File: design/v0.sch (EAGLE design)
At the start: 3 parts

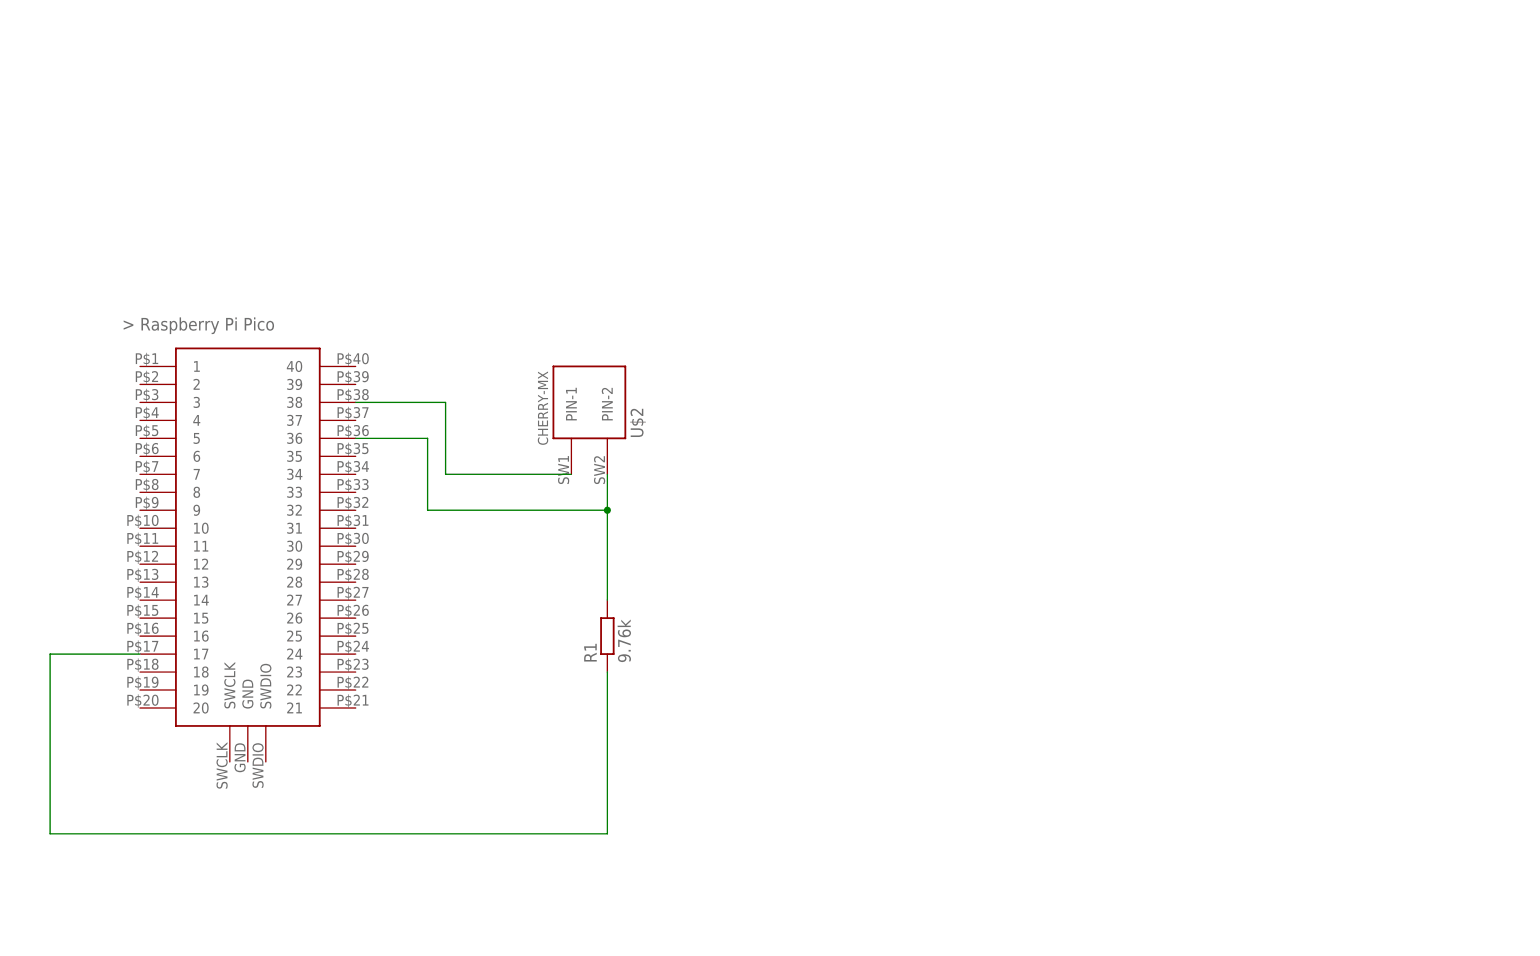
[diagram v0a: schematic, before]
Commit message: Update schematic
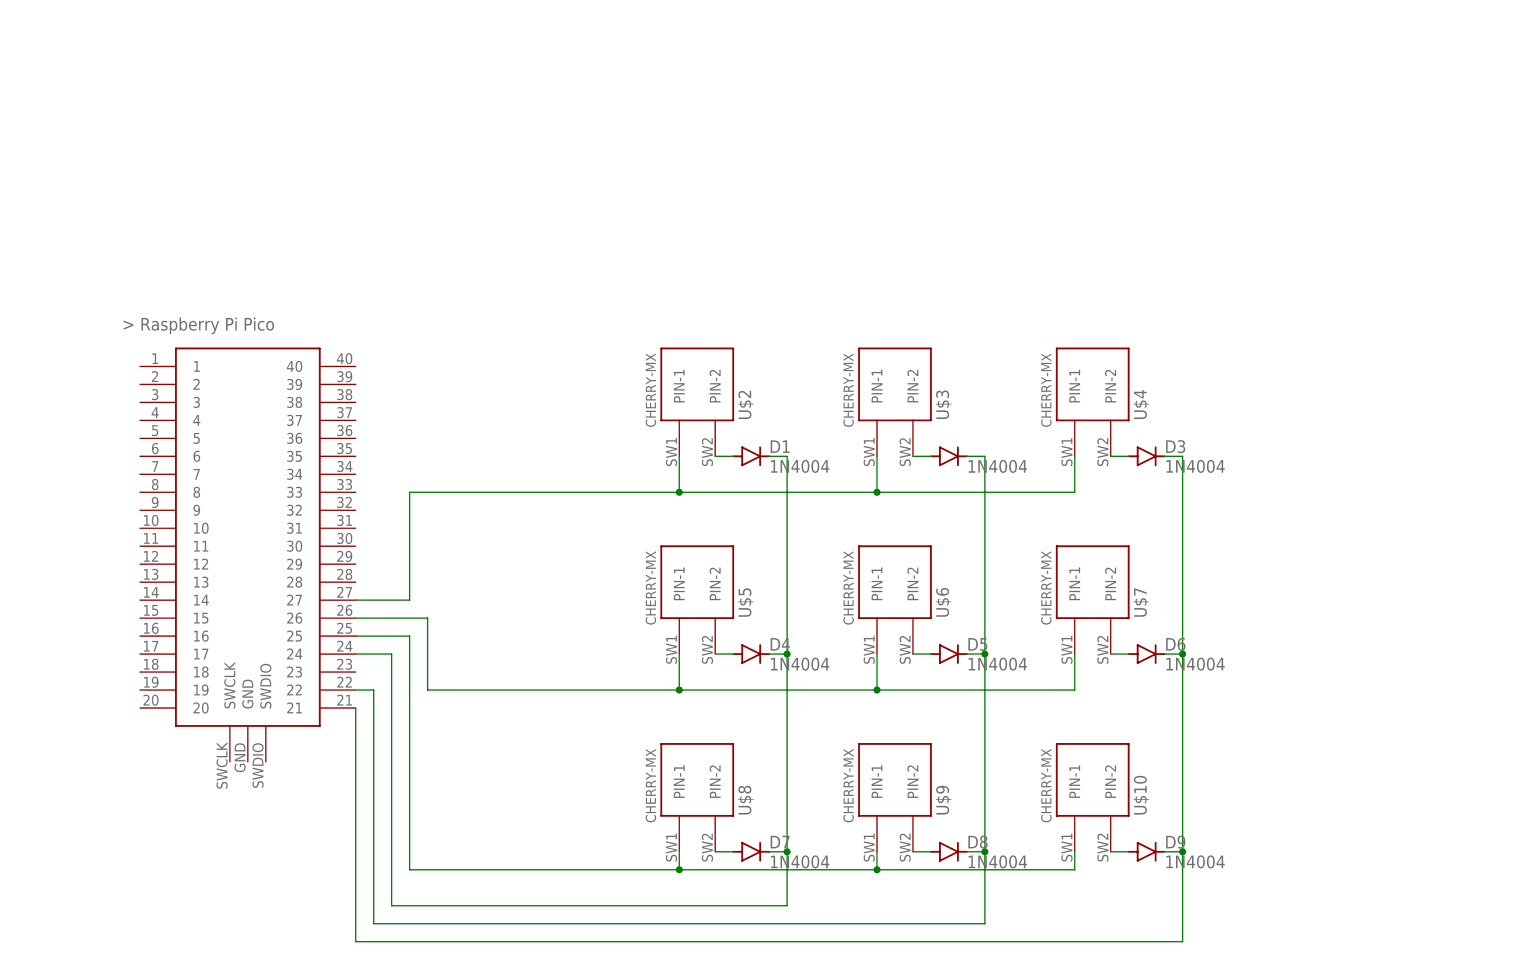
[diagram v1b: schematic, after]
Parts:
- removed R1: 9.76k, rcl:R-EU_0207/10
- added D1, D2, D3, D4, D5, D6, D7, D8, D9: 1N4004, diode:1N4004
- added U$10, U$3, U$4, U$5, U$6, U$7, U$8, U$9: CHERRY-MX, cherrymx:CHERRY-MX
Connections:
- new net N$10: D1.C, D4.C, D7.C, U$1.24
- new net N$11: D2.C, D5.C, D8.C, U$1.22
- new net N$12: D3.C, D6.C, D9.C, U$1.21
- new net N$13: U$1.27, U$2.PIN-1, U$3.PIN-1, U$4.PIN-1
- new net N$14: U$1.26, U$5.PIN-1, U$6.PIN-1, U$7.PIN-1
- new net N$15: U$1.25, U$10.PIN-1, U$8.PIN-1, U$9.PIN-1
- new net N$3: D3.A, U$4.PIN-2
- new net N$5: D5.A, U$6.PIN-2
- new net N$6: D6.A, U$7.PIN-2
- new net N$7: D9.A, U$10.PIN-2
- new net N$8: D8.A, U$9.PIN-2
- new net N$9: D7.A, U$8.PIN-2
- net N$1: now also D1.A, U$2.PIN-2; no longer U$1.38, U$2.PIN-1
- net N$2: now also D2.A, U$3.PIN-2; no longer R1.2, U$1.36, U$2.PIN-2
- net N$4: now also D4.A, U$5.PIN-2; no longer R1.1, U$1.17
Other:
- moved on the sheet: U$2

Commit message: Update schematic
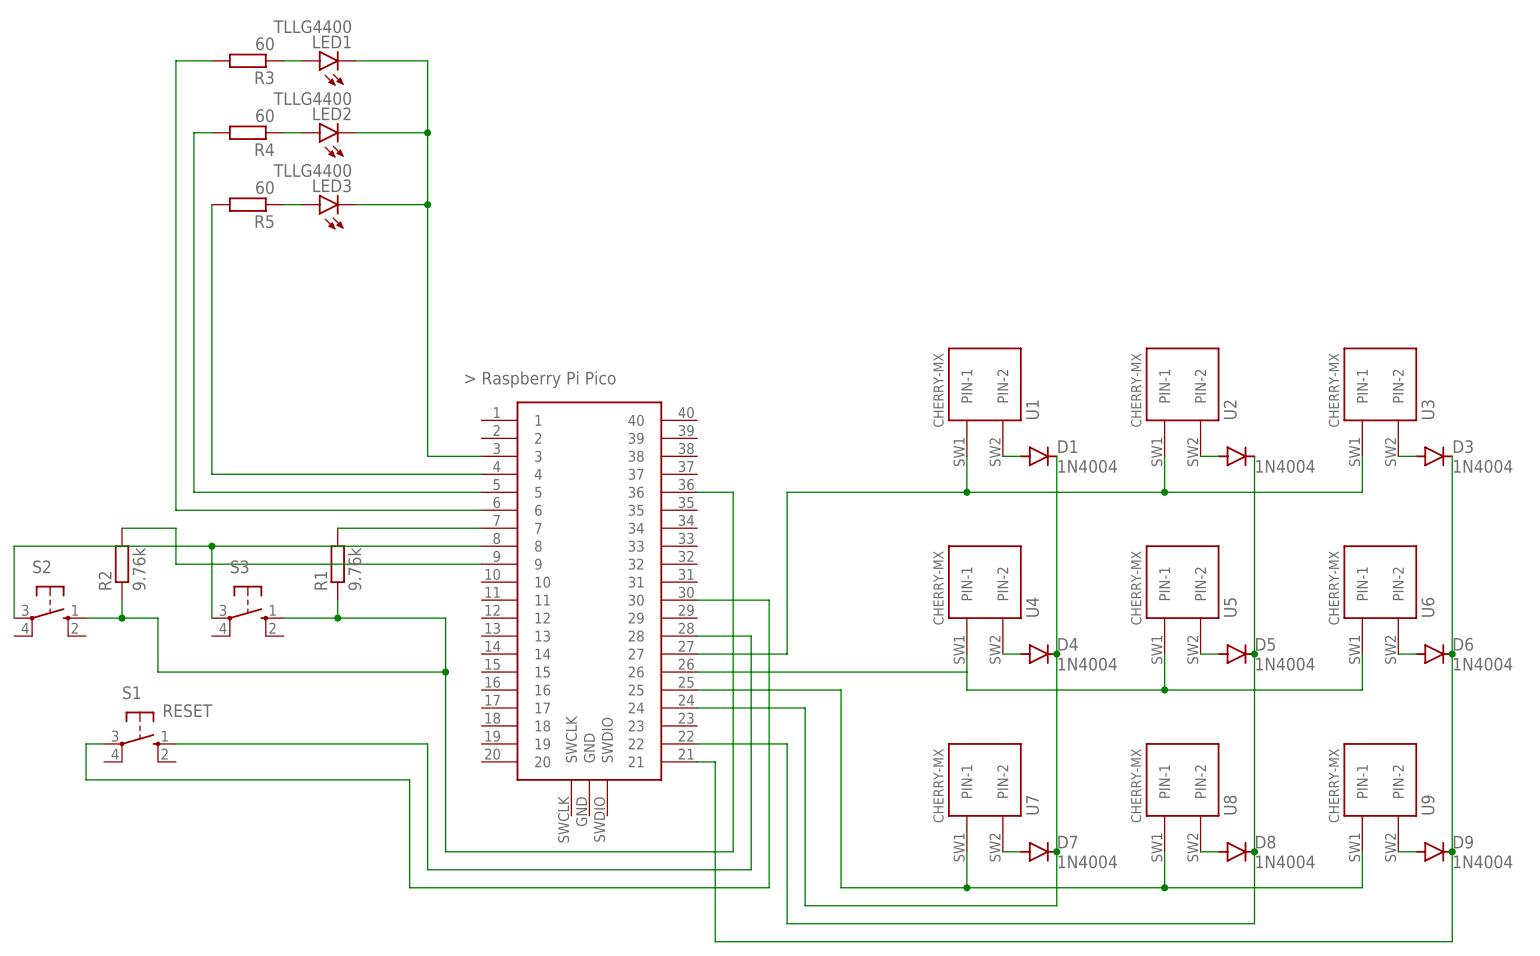
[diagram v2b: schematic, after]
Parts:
- removed U$10, U$2, U$3, U$4, U$5, U$6, U$7, U$8, U$9: CHERRY-MX, cherrymx:CHERRY-MX
- added LED1, LED2, LED3: TLLG4400, led:TLLG4400
- added R1, R2: 9.76k, rcl:R-EU_VMTA55
- added R3, R4, R5: 60, rcl:R-EU_VMTA55
- added S1: RESET, switch-omron:10-XX
- added S2, S3: (no value), switch-omron:10-XX
- added U1, U2, U3, U4, U5, U6, U7, U8, U9: CHERRY-MX, cherrymx:CHERRY-MX
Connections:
- removed net N$15 (its old number): U$1.25, U$10.PIN-1, U$8.PIN-1, U$9.PIN-1
- removed net N$8: D8.A, U$9.PIN-2
- new net N$10: R1.1, R2.1, S2.S, S3.S, U$1.36
- new net N$11: R2.2, U$1.9
- new net N$12: S2.P, S3.P, U$1.8
- new net N$18: D6.A, U6.PIN-2
- new net N$19: D3.A, U3.PIN-2
- new net N$20: D9.A, U9.PIN-2
- new net N$21: D8.A, U8.PIN-2
- new net N$22: D5.A, U5.PIN-2
- new net N$23: D2.A, U2.PIN-2
- new net N$24: D1.A, U1.PIN-2
- new net N$25: D4.A, U4.PIN-2
- new net N$26: D7.A, U7.PIN-2
- new net N$27: U$1.27, U1.PIN-1, U2.PIN-1, U3.PIN-1
- new net N$28: U$1.26, U4.PIN-1, U5.PIN-1, U6.PIN-1
- new net N$29: U$1.25, U7.PIN-1, U8.PIN-1, U9.PIN-1
- net N$1: now also LED2.A, R4.1; no longer D1.A, U$2.PIN-2
- net N$13: now also S1.S, U$1.28; no longer U$1.27, U$2.PIN-1, U$3.PIN-1, U$4.PIN-1
- net N$14: now also S1.P, U$1.30; no longer U$1.26, U$5.PIN-1, U$6.PIN-1, U$7.PIN-1
- net N$2: now also LED1.A, R3.1; no longer D2.A, U$3.PIN-2
- net N$3: now also LED3.A, R5.1; no longer D3.A, U$4.PIN-2
- net N$4: now also LED1.C, LED2.C, LED3.C, U$1.3; no longer D4.A, U$5.PIN-2
- net N$5: now also R5.2, U$1.4; no longer D5.A, U$6.PIN-2
- net N$6: now also R4.2, U$1.5; no longer D6.A, U$7.PIN-2
- net N$7: now also R3.2, U$1.6; no longer D9.A, U$10.PIN-2
- net N$9: now also R1.2, U$1.7; no longer D7.A, U$8.PIN-2
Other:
- moved on the sheet: D1, D3, D4, D5, D6, D7, D8, D9
